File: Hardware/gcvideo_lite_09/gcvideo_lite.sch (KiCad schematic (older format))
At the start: 42 parts, among them P1 Conn_01x16_Male, P2 Conn_01x03_Female, P3 Conn_01x03_Female, P4 Conn_01x04_Male, P5 Conn_01x02_Male, U1 MachXO2-256-TQ100, U2 ADV7125BCPZ170-RL, U4 74LVC14

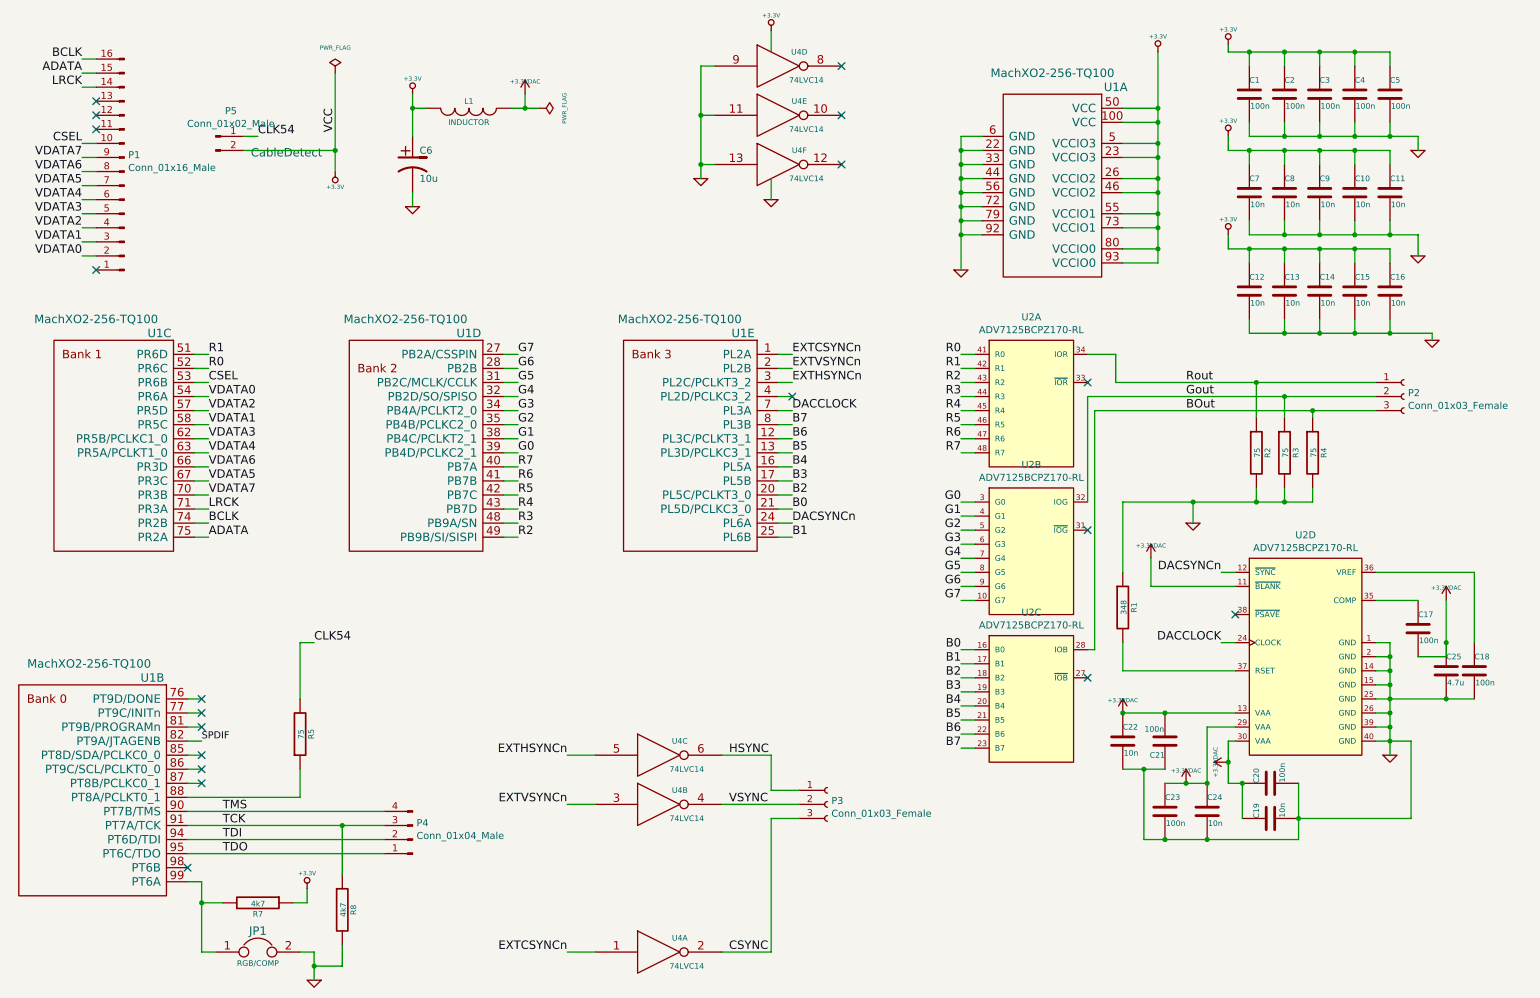
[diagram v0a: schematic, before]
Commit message: fully updated BOM
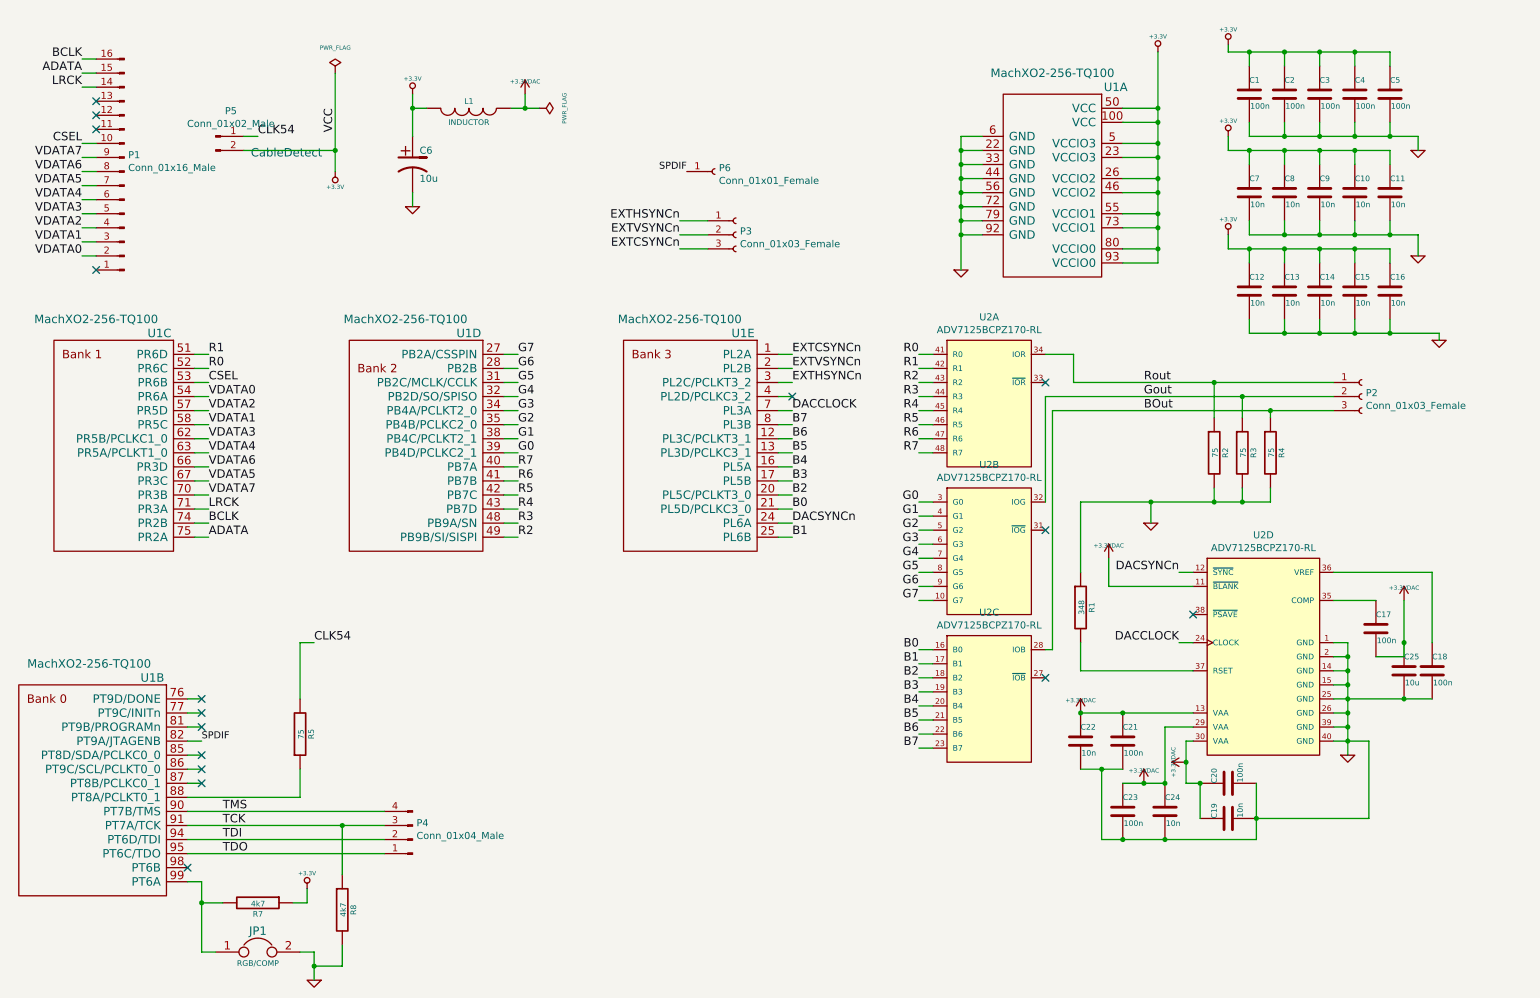
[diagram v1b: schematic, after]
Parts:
- removed U4: 74LVC14, Package_SO:SOIC-14_3.9x8.7mm_P1.27mm, symbol gcvideo_lite-rescue:74HC14
- added P6: Conn_01x01_Female, symbol Connector:Conn_01x01_Female
- C25: value 4.7u -> 10u
- C6: footprint Capacitor_SMD:C_1206_3216Metric_Pad1.33x1.80mm_HandSolder -> Capacitor_SMD:C_0805_2012Metric_Pad1.15x1.40mm_HandSolder
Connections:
- net CSYNC is gone; now on net EXTCSYNCn: P3.3 (Pin_3)
- net HSYNC is gone; now on net EXTHSYNCn: P3.1 (Pin_1)
- net VSYNC is gone; now on net EXTVSYNCn: P3.2 (Pin_2)
- net +3.3VDAC: now also C21.1; no longer C21.2
- net GND: now also C21.2; no longer C21.1
- net SPDIF: now also P6.1 (Pin_1)
- no-connect marks 19 -> 16
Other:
- moved on the sheet: C17, C18, C19, C20, C21, C22, C23, C24, C25, P2, P3, R1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
